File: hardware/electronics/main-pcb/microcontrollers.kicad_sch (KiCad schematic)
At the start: 34 parts, among them IC7 ATSAME53J18A-MF, U6 ATSAMD11D14A-M

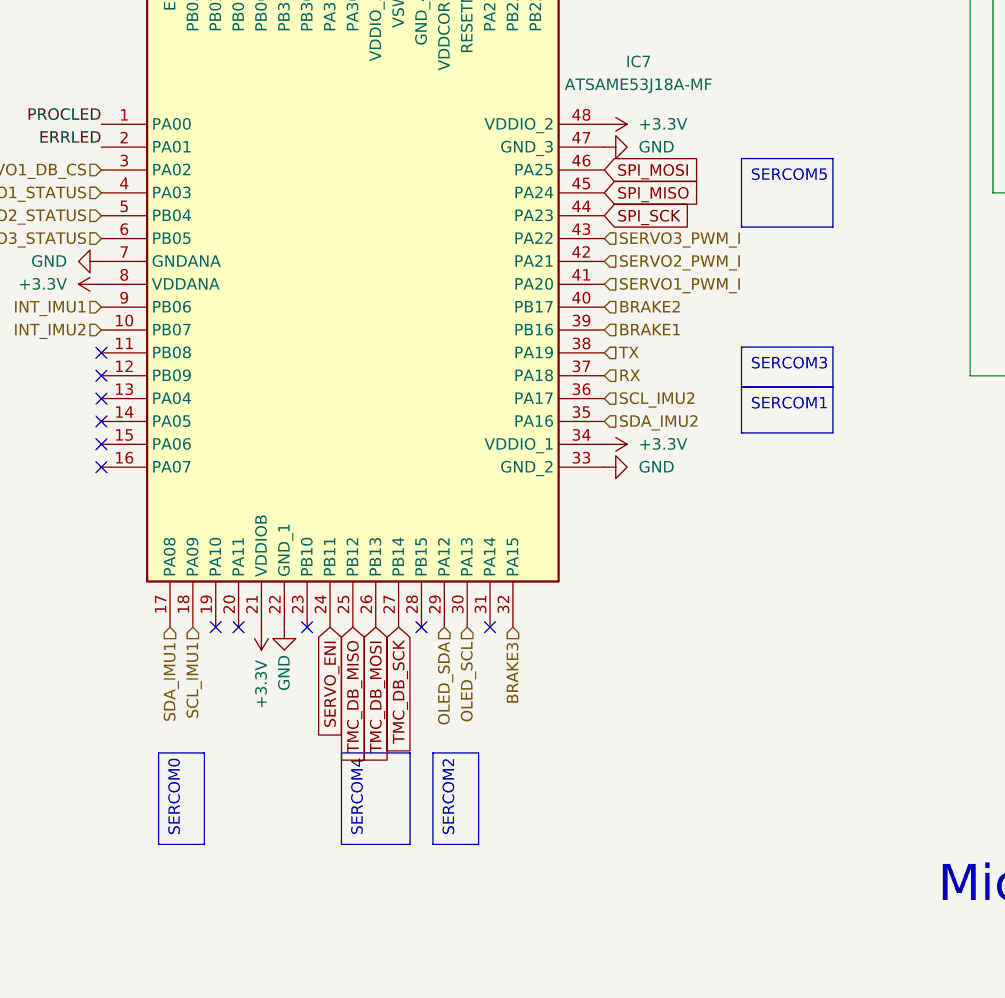
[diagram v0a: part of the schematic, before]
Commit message: wip
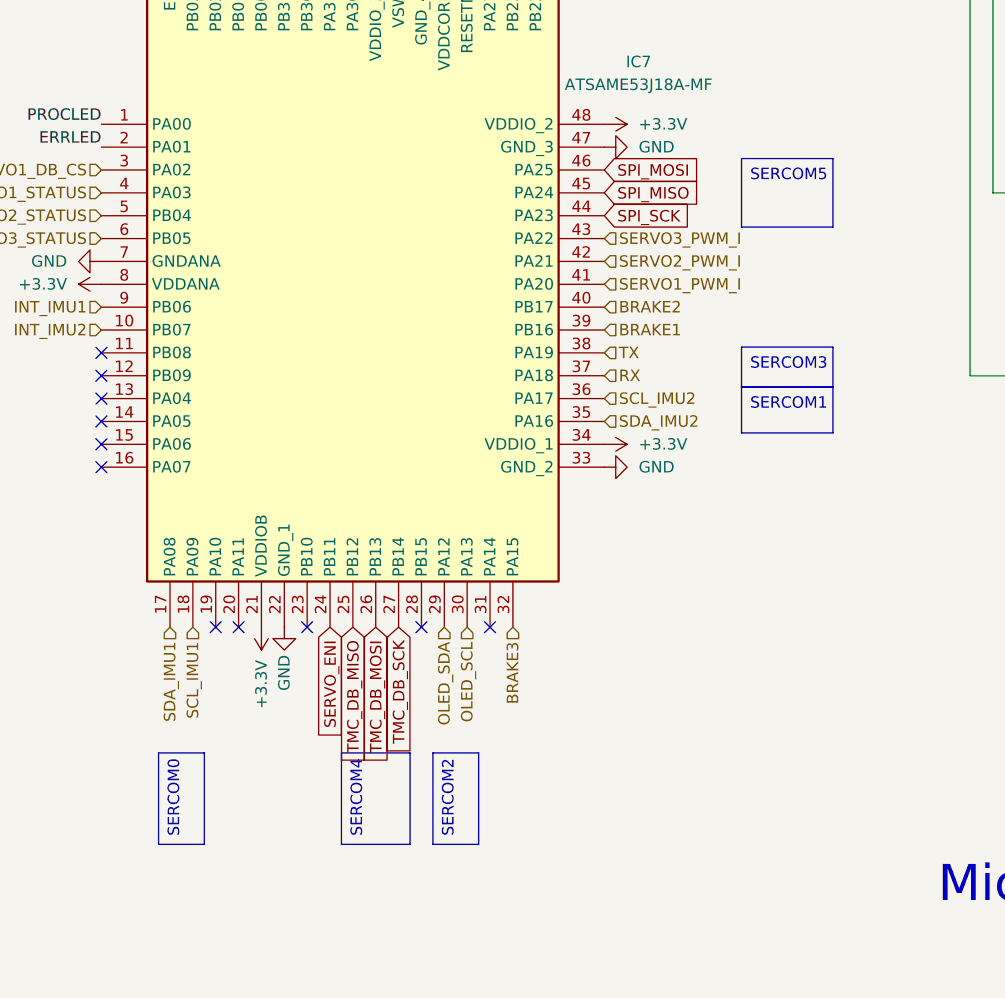
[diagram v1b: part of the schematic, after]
